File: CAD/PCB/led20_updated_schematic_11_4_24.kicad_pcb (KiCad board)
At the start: 2 copper layers, 55 x 55 mm, 32 parts, among them U6 B2B-PH-K-S, U7 B2B-PH-K-S

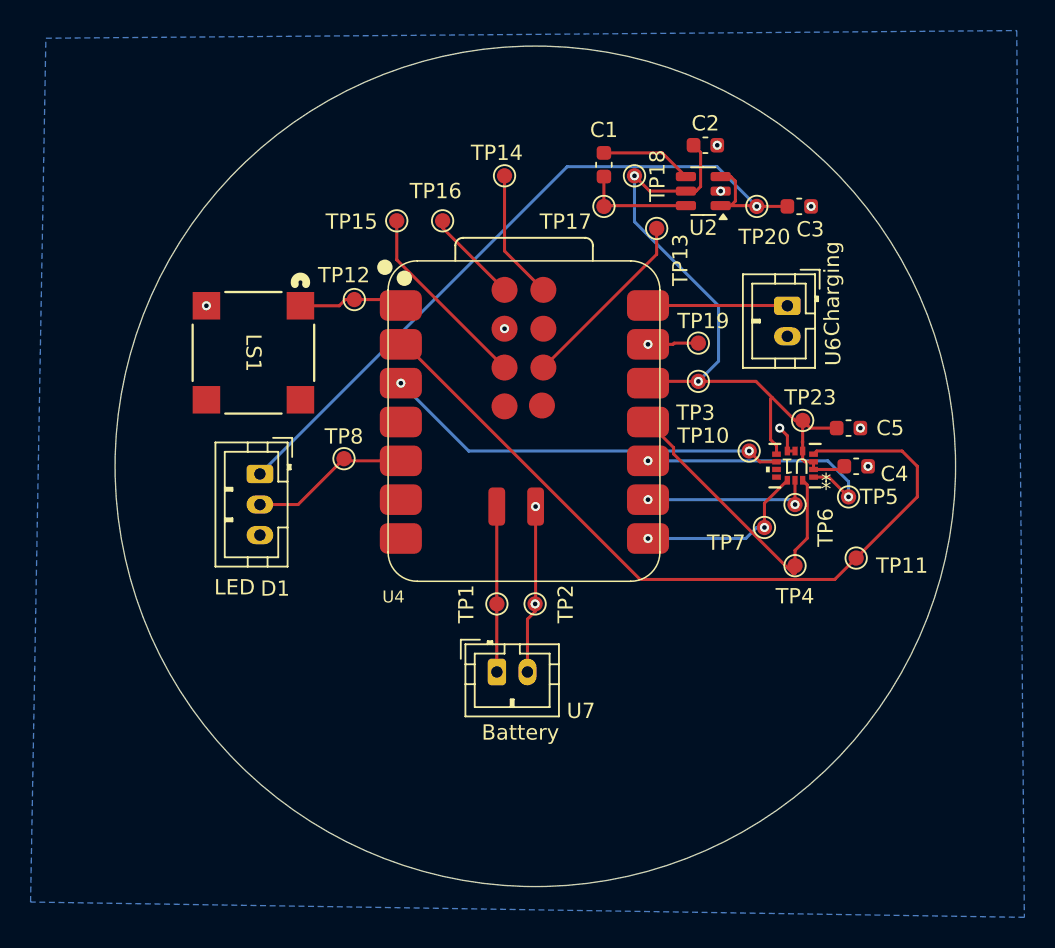
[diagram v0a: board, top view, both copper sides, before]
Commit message: PCB
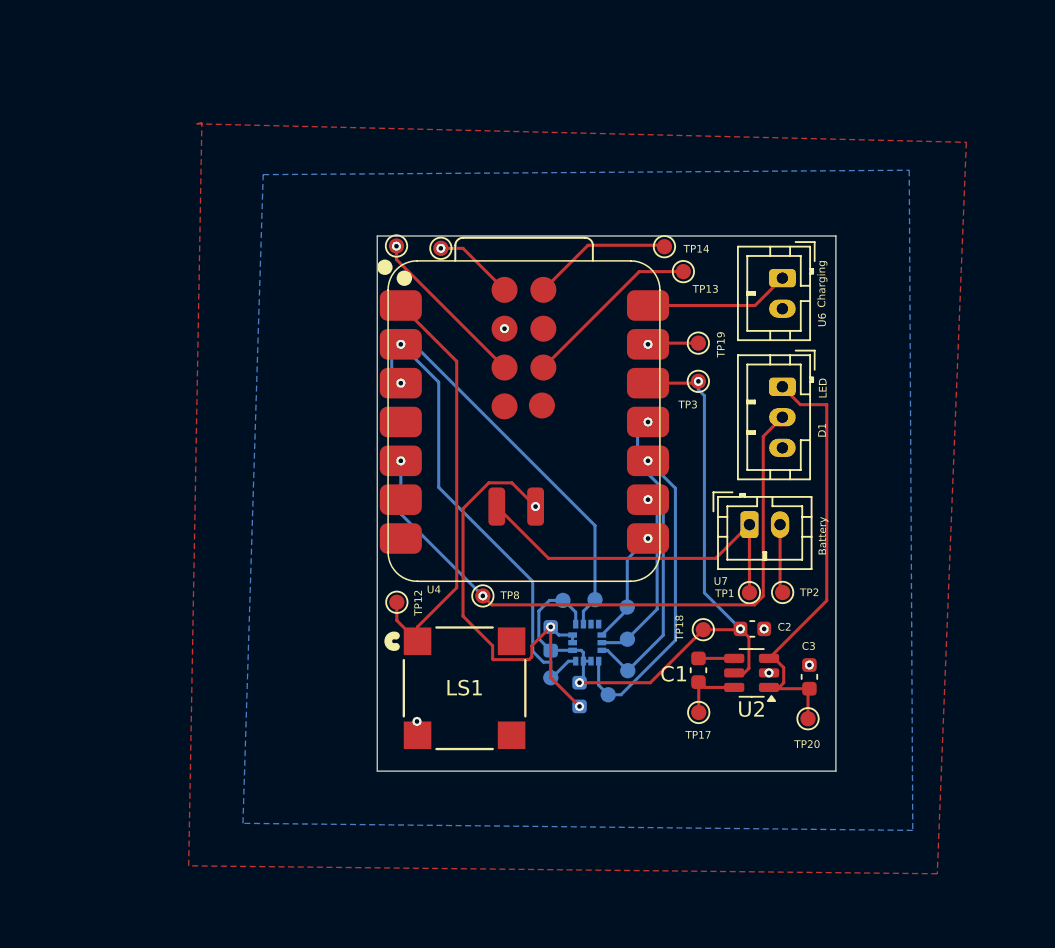
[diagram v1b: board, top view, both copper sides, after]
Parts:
- C4, C5, TP10, TP11, TP4, TP5, TP6, TP7, U1: moved to B.Cu
- TP21: renamed from TP23; moved to B.Cu
- moved D1 34.6 mm to (158.8, 73.2)
- moved TP20 33.7 mm to (160.5, 95.0)
- moved TP17 33.7 mm to (153.3, 94.5)
- moved C1 33.6 mm to (153.3, 91.8)
- moved C2 31.8 mm to (156.8, 89.1)
- moved U2 31.7 mm to (156.8, 92.0)
- moved C3 30.8 mm to (160.6, 92.2), turned to -90 degrees
- moved TP18 30.0 mm to (153.6, 89.1)
- moved LS1 25.9 mm to (138.0, 93.0), turned to 0 degrees
- moved C5 23.9 mm to (143.7, 89.7), turned to -90 degrees
- moved C4 23.5 mm to (145.5, 93.4), turned to 90 degrees
- moved TP11 21.5 mm to (143.7, 92.3), turned to -90 degrees
- moved TP5 20.4 mm to (147.4, 93.4), turned to -90 degrees
- moved TP12 20.0 mm to (133.6, 87.3)
- moved TP21 19.6 mm to (144.5, 87.2), turned to 90 degrees
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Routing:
- net 3.3V Data (D4): track 10.5 -> 42.1 mm, vias 0 -> 2
- net Net-(U1-INT1): track 51.7 -> 28.2 mm, vias 0 -> 1
- net Net-(U4-LP_GPIO0/GPIO0/A0/D0): track 6.90 -> 28.2 mm
- net GND: track 16.7 -> 37.9 mm, vias 11 -> 12
- net +5V: track 49.8 -> 29.5 mm, vias 1 -> 0
- net VBATT: track 10.8 -> 23.3 mm
- net Net-(U1-CS): track 11.7 -> 7.56 mm, vias 2 -> 1
- net Net-(U2-C-): track 6.00 -> 2.58 mm
- net Net-(U1-SDO/SA0): track 17.5 -> 20.8 mm, vias 2 -> 1
- net Net-(U2-C+): track 7.26 -> 4.47 mm
- net Net-(U1-INT2): track 26.7 -> 28.4 mm, vias 2 -> 1
- net unconnected-(TP15-Pad1): track 12.5 -> 10.9 mm, vias 0 -> 1
- net unconnected-(TP16-Pad1): track 6.20 -> 5.29 mm, vias 0 -> 1
- net unconnected-(TP14-Pad1): track 8.51 -> 9.17 mm
- net 3.3V: track 47.6 -> 48.3 mm, vias 2 -> 3
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- added copper zone on F.Cu, net GND
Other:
- board size 55 x 55 mm -> 30 x 35 mm
